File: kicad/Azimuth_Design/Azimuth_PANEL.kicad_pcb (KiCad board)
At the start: 4 copper layers, 101 x 58 mm, 344 parts, among them IC1 BNO086, J1 TYPE-C 16PIN 2MD(073), Q1 LP0404N3T5G, Q2 AO3400A, Q3 AO3401A, U1 ESP32-C3-WROOM-02-N4(4MB), U2 TLV75733PDBVR, U3 TP4054_C5381776

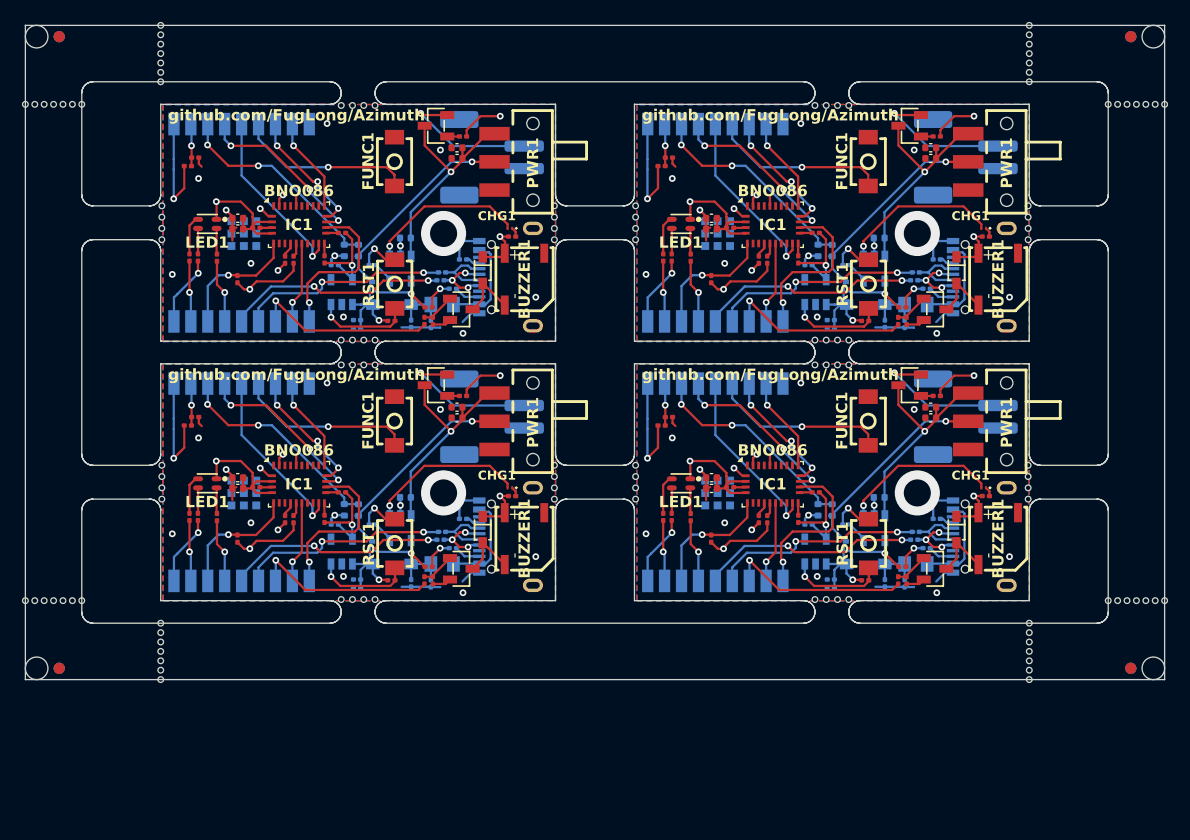
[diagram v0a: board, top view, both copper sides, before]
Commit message: PCB V0.1 ordered!
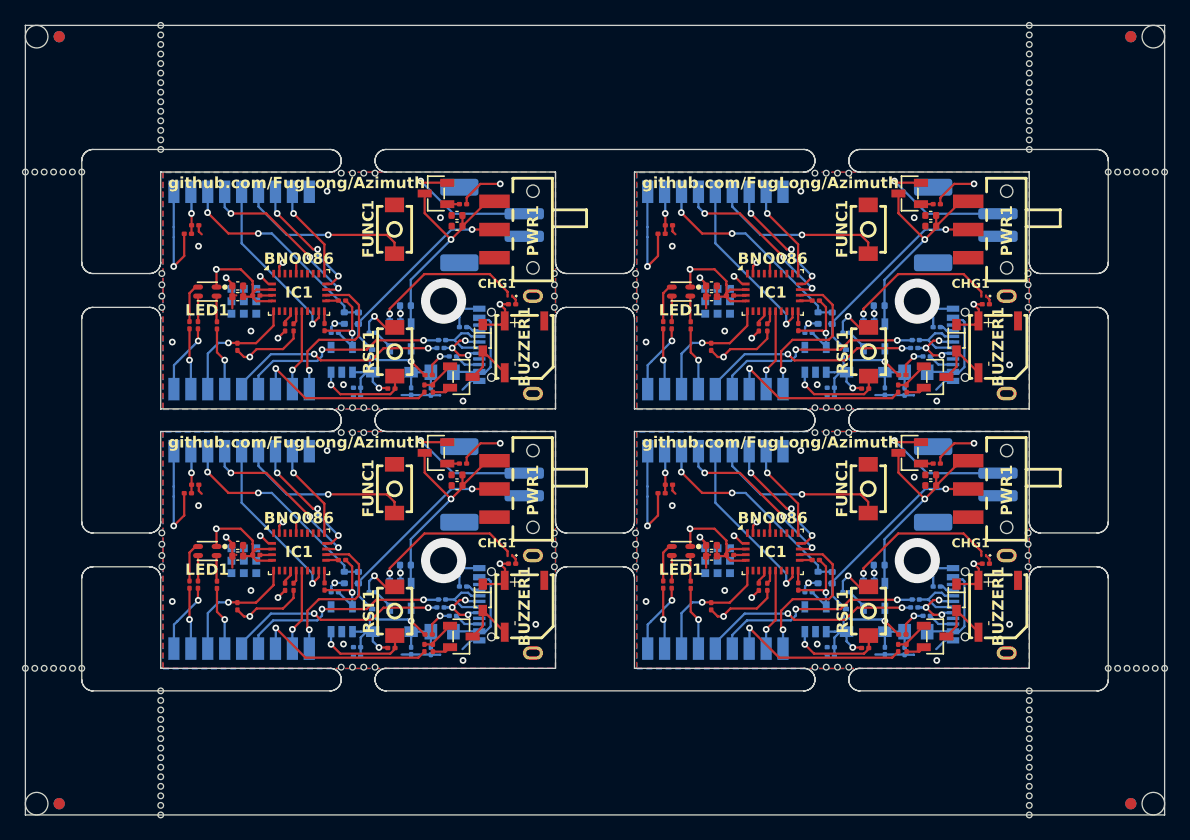
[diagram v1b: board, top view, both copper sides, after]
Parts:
- removed the BUZZER1 at (184.2, 42.5)
- removed the BUZZER1 at (184.2, 65.5)
- removed the BUZZER1 at (142.2, 42.5)
- removed the BUZZER1 at (142.2, 65.5)
- removed the C1 at (136.3, 53.9)
- removed the C1 at (178.3, 30.9)
- removed the C1 at (136.3, 30.9)
- removed the C1 at (178.3, 53.9)
- removed the C10 at (158.8, 61.0)
- removed the C10 at (116.8, 38.0)
- removed the C10 at (158.8, 38.0)
- removed the C10 at (116.8, 61.0)
- removed the C11 at (163.0, 63.8)
- removed the C11 at (121.0, 63.8)
- removed the C11 at (121.0, 40.8)
- removed the C11 at (163.0, 40.8)
- removed the C12 at (113.1, 54.7)
- removed the C12 at (113.1, 31.7)
- removed the C12 at (155.1, 54.7)
- removed the C12 at (155.1, 31.7)
- removed the C2 at (136.3, 31.8)
- removed the C2 at (136.3, 54.8)
- removed the C2 at (178.3, 54.8)
- removed the C2 at (178.3, 31.8)
- removed the C3 at (175.9, 69.5)
- removed the C3 at (133.9, 46.5)
- removed the C3 at (175.9, 46.5)
- removed the C3 at (133.9, 69.5)
- removed the C4 at (127.4, 69.1)
- removed the C4 at (169.4, 46.1)
- removed the C4 at (127.4, 46.1)
- removed the C4 at (169.4, 69.1)
- removed the C5 at (127.4, 46.9)
- removed the C5 at (169.4, 69.9)
- removed the C5 at (169.4, 46.9)
- removed the C5 at (127.4, 69.9)
- removed the C6 at (125.4, 64.2)
- removed the C6 at (125.4, 41.2)
- removed the C6 at (167.4, 41.2)
- removed the C6 at (167.4, 64.2)
- removed the C7 at (133.8, 45.0)
- removed the C7 at (133.8, 68.0)
- removed the C7 at (175.8, 45.0)
- removed the C7 at (175.8, 68.0)
- removed the C8 at (173.7, 38.9)
- removed the C8 at (131.7, 38.9)
- removed the C8 at (131.7, 61.9)
- removed the C8 at (173.7, 61.9)
- removed the C9 at (116.8, 37.1)
- removed the C9 at (116.8, 60.1)
- removed the C9 at (158.8, 37.1)
- removed the C9 at (158.8, 60.1)
- removed the CHG1 at (140.9, 61.0)
- removed the CHG1 at (182.9, 61.0)
- removed the CHG1 at (140.9, 38.0)
- removed the CHG1 at (182.9, 38.0)
- removed the D1 at (172.5, 44.8)
- removed the D1 at (130.5, 67.8)
- removed the D1 at (130.5, 44.8)
- removed the D1 at (172.5, 67.8)
- removed the D2 at (180.6, 64.7)
- removed the D2 at (138.6, 41.7)
- removed the D2 at (138.6, 64.7)
- removed the D2 at (180.6, 41.7)
- removed the F1 at (134.9, 44.8)
- removed the F1 at (176.9, 67.8)
- removed the F1 at (176.9, 44.8)
- removed the F1 at (134.9, 67.8)
- removed the FUNC1 at (130.7, 32.1)
- removed the FUNC1 at (172.7, 55.1)
- removed the FUNC1 at (172.7, 32.1)
- removed the FUNC1 at (130.7, 55.1)
- removed the G*** at (171.1, 55.7)
- removed the G*** at (129.1, 32.7)
- removed the G*** at (171.1, 32.7)
- removed the G*** at (129.1, 55.7)
- removed the IC1 at (164.3, 37.7)
- removed the IC1 at (164.3, 60.7)
- removed the IC1 at (122.3, 37.7)
- removed the IC1 at (122.3, 60.7)
- removed the J1 at (140.6, 42.3)
- removed the J1 at (182.6, 65.3)
- removed the J1 at (182.6, 42.3)
- removed the J1 at (140.6, 65.3)
- removed the LED1 at (156.1, 37.6)
- removed the LED1 at (114.1, 37.6)
- removed the LED1 at (114.1, 60.6)
- removed the LED1 at (156.1, 60.6)
- removed the PH2.0 at (181.4, 54.7)
- removed the PH2.0 at (139.4, 54.7)
- removed the PH2.0 at (181.4, 31.7)
- removed the PH2.0 at (139.4, 31.7)
- removed the PWR1 at (139.6, 32.1)
- removed the PWR1 at (181.6, 55.1)
- removed the PWR1 at (181.6, 32.1)
- removed the PWR1 at (139.6, 55.1)
- removed the Q1 at (128.8, 43.1)
- removed the Q1 at (170.8, 66.1)
- removed the Q1 at (170.8, 43.1)
- removed the Q1 at (128.8, 66.1)
- removed the Q2 at (178.7, 68.2)
- removed the Q2 at (178.7, 45.2)
- removed the Q2 at (136.7, 68.2)
- removed the Q2 at (136.7, 45.2)
- removed the Q3 at (176.4, 51.9)
- removed the Q3 at (134.4, 51.9)
- removed the Q3 at (134.4, 28.9)
- removed the Q3 at (176.4, 28.9)
- removed the R1 at (168.3, 40.0)
- removed the R1 at (168.3, 63.0)
- removed the R1 at (126.3, 63.0)
- removed the R1 at (126.3, 40.0)
- removed the R10 at (135.9, 66.3)
- removed the R10 at (135.9, 43.4)
- removed the R10 at (177.9, 43.4)
- removed the R10 at (177.9, 66.3)
- removed the R11 at (176.8, 42.6)
- removed the R11 at (134.8, 42.6)
- removed the R11 at (176.8, 65.6)
- removed the R11 at (134.8, 65.6)
- removed the R12 at (176.9, 41.9)
- removed the R12 at (176.9, 64.9)
- removed the R12 at (134.9, 64.9)
- removed the R12 at (134.9, 41.9)
- removed the R13 at (118.5, 38.0)
- removed the R13 at (118.5, 61.0)
- removed the R13 at (160.5, 38.0)
- removed the R13 at (160.5, 61.0)
- removed the R14 at (116.8, 65.5)
- removed the R14 at (158.8, 42.5)
- removed the R14 at (116.8, 42.5)
- removed the R14 at (158.8, 65.5)
- removed the R15 at (121.8, 63.8)
- removed the R15 at (163.8, 40.8)
- removed the R15 at (121.8, 40.8)
- removed the R15 at (163.8, 63.8)
- removed the R16 at (166.5, 40.8)
- removed the R16 at (166.5, 63.8)
- removed the R16 at (124.5, 63.8)
- removed the R16 at (124.5, 40.8)
- removed the R17 at (126.1, 38.4)
- removed the R17 at (168.1, 38.4)
- removed the R17 at (126.1, 61.4)
- removed the R17 at (168.1, 61.4)
- removed the R18 at (154.4, 32.5)
- removed the R18 at (112.4, 55.5)
- removed the R18 at (154.4, 55.5)
- removed the R18 at (112.4, 32.5)
- removed the R19 at (172.4, 69.2)
- removed the R19 at (172.4, 46.2)
- removed the R19 at (130.4, 46.2)
- removed the R19 at (130.4, 69.2)
- removed the R2 at (169.5, 40.0)
- removed the R2 at (169.5, 63.0)
- removed the R2 at (127.5, 63.0)
- removed the R2 at (127.5, 40.0)
- removed the R20 at (175.4, 46.2)
- removed the R20 at (133.4, 46.2)
- removed the R20 at (175.4, 69.2)
- removed the R20 at (133.4, 69.2)
- removed the R21 at (176.1, 46.2)
- removed the R21 at (134.1, 69.2)
- removed the R21 at (176.1, 69.2)
- removed the R21 at (134.1, 46.2)
- removed the R22 at (136.8, 29.9)
- removed the R22 at (178.8, 29.9)
- removed the R22 at (136.8, 52.9)
- removed the R22 at (178.8, 52.9)
- removed the R3 at (132.2, 69.5)
- removed the R3 at (174.2, 46.5)
- removed the R3 at (132.2, 46.5)
- removed the R3 at (174.2, 69.5)
- removed the R4 at (170.8, 41.2)
- removed the R4 at (128.8, 41.2)
- removed the R4 at (170.8, 64.2)
- removed the R4 at (128.8, 64.2)
- removed the R5 at (183.2, 38.7)
- removed the R5 at (183.2, 61.7)
- removed the R5 at (141.2, 61.7)
- removed the R5 at (141.2, 38.7)
- removed the R6 at (157.0, 40.6)
- removed the R6 at (115.0, 40.6)
- removed the R6 at (115.0, 63.6)
- removed the R6 at (157.0, 63.6)
- removed the R7 at (113.3, 40.6)
- removed the R7 at (155.3, 40.6)
- removed the R7 at (113.3, 63.6)
- removed the R7 at (155.3, 63.6)
- removed the R8 at (112.5, 40.6)
- removed the R8 at (112.5, 63.6)
- removed the R8 at (154.6, 63.6)
- removed the R8 at (154.6, 40.6)
- removed the R9 at (178.8, 40.8)
- removed the R9 at (136.8, 40.8)
- removed the R9 at (136.8, 63.8)
- removed the R9 at (178.8, 63.8)
- removed the RST1 at (130.8, 65.9)
- removed the RST1 at (130.8, 42.9)
- removed the RST1 at (172.8, 42.9)
- removed the RST1 at (172.8, 65.9)
- removed the U1 at (117.2, 60.5)
- removed the U1 at (159.2, 37.5)
- removed the U1 at (117.2, 37.5)
- removed the U1 at (159.2, 60.5)
- removed the U2 at (168.1, 43.6)
- removed the U2 at (126.0, 66.7)
- removed the U2 at (168.1, 66.7)
- removed the U2 at (126.0, 43.6)
- removed the U3 at (173.2, 41.6)
- removed the U3 at (131.2, 64.6)
- removed the U3 at (173.2, 64.6)
- removed the U3 at (131.2, 41.6)
- added BUZZER1: MLT-5020, 1_MyFootPrints:BUZ-SMD_L5.0-W5.5-P4.60, F.Cu at (184.2, 71.5)
- added BUZZER1: MLT-5020, 1_MyFootPrints:BUZ-SMD_L5.0-W5.5-P4.60, F.Cu at (184.2, 48.5)
- added BUZZER1: MLT-5020, 1_MyFootPrints:BUZ-SMD_L5.0-W5.5-P4.60, F.Cu at (142.2, 71.5)
- added BUZZER1: MLT-5020, 1_MyFootPrints:BUZ-SMD_L5.0-W5.5-P4.60, F.Cu at (142.2, 48.5)
- added C1: 10uf, Capacitor_SMD:C_0402_1005Metric, F.Cu at (178.3, 36.9)
- added C1: 10uf, Capacitor_SMD:C_0402_1005Metric, F.Cu at (136.3, 36.9)
- added C1: 10uf, Capacitor_SMD:C_0402_1005Metric, F.Cu at (136.3, 59.9)
- added C1: 10uf, Capacitor_SMD:C_0402_1005Metric, F.Cu at (178.3, 59.9)
- added C10: 0.1uf, Capacitor_SMD:C_0402_1005Metric, F.Cu at (158.8, 44.0)
- added C10: 0.1uf, Capacitor_SMD:C_0402_1005Metric, F.Cu at (116.8, 67.0)
- added C10: 0.1uf, Capacitor_SMD:C_0402_1005Metric, F.Cu at (116.8, 44.0)
- added C10: 0.1uf, Capacitor_SMD:C_0402_1005Metric, F.Cu at (158.8, 67.0)
- added C11: 100nf, Capacitor_SMD:C_0201_0603Metric, F.Cu at (163.0, 46.8)
- added C11: 100nf, Capacitor_SMD:C_0201_0603Metric, F.Cu at (121.0, 69.8)
- added C11: 100nf, Capacitor_SMD:C_0201_0603Metric, F.Cu at (163.0, 69.8)
- added C11: 100nf, Capacitor_SMD:C_0201_0603Metric, F.Cu at (121.0, 46.8)
- added C12: 100nf, Capacitor_SMD:C_0201_0603Metric, F.Cu at (155.1, 37.7)
- added C12: 100nf, Capacitor_SMD:C_0201_0603Metric, F.Cu at (155.1, 60.7)
- added C12: 100nf, Capacitor_SMD:C_0201_0603Metric, F.Cu at (113.1, 60.7)
- added C12: 100nf, Capacitor_SMD:C_0201_0603Metric, F.Cu at (113.1, 37.7)
- added C2: 0.1uf, Capacitor_SMD:C_0402_1005Metric, F.Cu at (178.3, 37.8)
- added C2: 0.1uf, Capacitor_SMD:C_0402_1005Metric, F.Cu at (136.3, 60.8)
- added C2: 0.1uf, Capacitor_SMD:C_0402_1005Metric, F.Cu at (178.3, 60.8)
- added C2: 0.1uf, Capacitor_SMD:C_0402_1005Metric, F.Cu at (136.3, 37.8)
- added C3: 100nf, Capacitor_SMD:C_0201_0603Metric, B.Cu at (175.9, 52.5)
- added C3: 100nf, Capacitor_SMD:C_0201_0603Metric, B.Cu at (133.9, 52.5)
- added C3: 100nf, Capacitor_SMD:C_0201_0603Metric, B.Cu at (175.9, 75.5)
- added C3: 100nf, Capacitor_SMD:C_0201_0603Metric, B.Cu at (133.9, 75.5)
- added C4: 2.2uf, Capacitor_SMD:C_0201_0603Metric, B.Cu at (127.4, 52.1)
- added C4: 2.2uf, Capacitor_SMD:C_0201_0603Metric, B.Cu at (169.4, 52.1)
- added C4: 2.2uf, Capacitor_SMD:C_0201_0603Metric, B.Cu at (169.4, 75.1)
- added C4: 2.2uf, Capacitor_SMD:C_0201_0603Metric, B.Cu at (127.4, 75.1)
- added C5: 2.2uf, Capacitor_SMD:C_0201_0603Metric, B.Cu at (127.4, 75.9)
- added C5: 2.2uf, Capacitor_SMD:C_0201_0603Metric, B.Cu at (127.4, 52.9)
- added C5: 2.2uf, Capacitor_SMD:C_0201_0603Metric, B.Cu at (169.4, 52.9)
- added C5: 2.2uf, Capacitor_SMD:C_0201_0603Metric, B.Cu at (169.4, 75.9)
- added C6: 2.2uf, Capacitor_SMD:C_0201_0603Metric, B.Cu at (125.4, 47.2)
- added C6: 2.2uf, Capacitor_SMD:C_0201_0603Metric, B.Cu at (167.4, 70.2)
- added C6: 2.2uf, Capacitor_SMD:C_0201_0603Metric, B.Cu at (125.4, 70.2)
- added C6: 2.2uf, Capacitor_SMD:C_0201_0603Metric, B.Cu at (167.4, 47.2)
- added C7: 2.2uf, Capacitor_SMD:C_0201_0603Metric, F.Cu at (175.8, 74.0)
- added C7: 2.2uf, Capacitor_SMD:C_0201_0603Metric, F.Cu at (175.8, 51.0)
- added C7: 2.2uf, Capacitor_SMD:C_0201_0603Metric, F.Cu at (133.8, 74.0)
- added C7: 2.2uf, Capacitor_SMD:C_0201_0603Metric, F.Cu at (133.8, 51.0)
- added C8: 10uf, Capacitor_SMD:C_0402_1005Metric, B.Cu at (173.7, 67.8)
- added C8: 10uf, Capacitor_SMD:C_0402_1005Metric, B.Cu at (131.7, 44.9)
- added C8: 10uf, Capacitor_SMD:C_0402_1005Metric, B.Cu at (131.7, 67.8)
- added C8: 10uf, Capacitor_SMD:C_0402_1005Metric, B.Cu at (173.7, 44.9)
- added C9: 10uf, Capacitor_SMD:C_0402_1005Metric, F.Cu at (158.8, 43.1)
- added C9: 10uf, Capacitor_SMD:C_0402_1005Metric, F.Cu at (116.8, 66.1)
- added C9: 10uf, Capacitor_SMD:C_0402_1005Metric, F.Cu at (116.8, 43.1)
- added C9: 10uf, Capacitor_SMD:C_0402_1005Metric, F.Cu at (158.8, 66.1)
- added CHG1: XL-0201SURC, 1_MyFootPrints:LED-SMD_L0.65-W0.35-P0.41_XL-0201SURC, F.Cu at (182.9, 44.0)
- added CHG1: XL-0201SURC, 1_MyFootPrints:LED-SMD_L0.65-W0.35-P0.41_XL-0201SURC, F.Cu at (182.9, 67.0)
- added CHG1: XL-0201SURC, 1_MyFootPrints:LED-SMD_L0.65-W0.35-P0.41_XL-0201SURC, F.Cu at (140.9, 67.0)
- added CHG1: XL-0201SURC, 1_MyFootPrints:LED-SMD_L0.65-W0.35-P0.41_XL-0201SURC, F.Cu at (140.9, 44.0)
- added D1: MBR0530_C5204746, 1_MyFootPrints:SOD-123_L2.7-W1.6-LS3.7-RD-1, B.Cu at (172.5, 50.8)
- added D1: MBR0530_C5204746, 1_MyFootPrints:SOD-123_L2.7-W1.6-LS3.7-RD-1, B.Cu at (130.5, 73.8)
- added D1: MBR0530_C5204746, 1_MyFootPrints:SOD-123_L2.7-W1.6-LS3.7-RD-1, B.Cu at (172.5, 73.8)
- added D1: MBR0530_C5204746, 1_MyFootPrints:SOD-123_L2.7-W1.6-LS3.7-RD-1, B.Cu at (130.5, 50.8)
- added D2: B5819WS, 1_MyFootPrints:SOD-323_L1.8-W1.3-LS2.5-RD, F.Cu at (180.6, 70.7)
- added D2: B5819WS, 1_MyFootPrints:SOD-323_L1.8-W1.3-LS2.5-RD, F.Cu at (138.6, 47.7)
- added D2: B5819WS, 1_MyFootPrints:SOD-323_L1.8-W1.3-LS2.5-RD, F.Cu at (180.6, 47.7)
- added D2: B5819WS, 1_MyFootPrints:SOD-323_L1.8-W1.3-LS2.5-RD, F.Cu at (138.6, 70.7)
- added F1: 0805L050WR, 1_MyFootPrints:R0805, B.Cu at (176.9, 73.8)
- added F1: 0805L050WR, 1_MyFootPrints:R0805, B.Cu at (176.9, 50.8)
- added F1: 0805L050WR, 1_MyFootPrints:R0805, B.Cu at (134.9, 73.8)
- added F1: 0805L050WR, 1_MyFootPrints:R0805, B.Cu at (134.9, 50.8)
- added FUNC1: HX 3X4X2-2P-1.6N TACTILE SWITCH, 1_MyFootPrints:KEY-SMD_L4.0-W3.0-LS4.9-1, F.Cu at (172.7, 38.1)
- added FUNC1: HX 3X4X2-2P-1.6N TACTILE SWITCH, 1_MyFootPrints:KEY-SMD_L4.0-W3.0-LS4.9-1, F.Cu at (130.7, 61.1)
- added FUNC1: HX 3X4X2-2P-1.6N TACTILE SWITCH, 1_MyFootPrints:KEY-SMD_L4.0-W3.0-LS4.9-1, F.Cu at (130.7, 38.1)
- added FUNC1: HX 3X4X2-2P-1.6N TACTILE SWITCH, 1_MyFootPrints:KEY-SMD_L4.0-W3.0-LS4.9-1, F.Cu at (172.7, 61.1)
- added G***: LOGO, LOGO, B.Cu at (129.1, 38.7)
- added G***: LOGO, LOGO, B.Cu at (129.1, 61.7)
- added G***: LOGO, LOGO, B.Cu at (171.1, 38.7)
- added G***: LOGO, LOGO, B.Cu at (171.1, 61.7)
- added IC1: BNO086, Package_LGA:LGA-28_5.2x3.8mm_P0.5mm, F.Cu at (164.3, 66.7)
- added IC1: BNO086, Package_LGA:LGA-28_5.2x3.8mm_P0.5mm, F.Cu at (122.3, 43.7)
- added IC1: BNO086, Package_LGA:LGA-28_5.2x3.8mm_P0.5mm, F.Cu at (122.3, 66.7)
- added IC1: BNO086, Package_LGA:LGA-28_5.2x3.8mm_P0.5mm, F.Cu at (164.3, 43.7)
- added J1: TYPE-C 16PIN 2MD(073), 1_MyFootPrints:USB-C-SMD_TYPE-C-6PIN-2MD-073, B.Cu at (140.6, 71.3)
- added J1: TYPE-C 16PIN 2MD(073), 1_MyFootPrints:USB-C-SMD_TYPE-C-6PIN-2MD-073, B.Cu at (182.6, 48.3)
- added J1: TYPE-C 16PIN 2MD(073), 1_MyFootPrints:USB-C-SMD_TYPE-C-6PIN-2MD-073, B.Cu at (182.6, 71.3)
- added J1: TYPE-C 16PIN 2MD(073), 1_MyFootPrints:USB-C-SMD_TYPE-C-6PIN-2MD-073, B.Cu at (140.6, 48.3)
- added KiKit_MB_17_10: NPTH, NPTH, F.Cu at (110.0, 27.6)
- added KiKit_MB_17_11: NPTH, NPTH, F.Cu at (110.0, 28.5)
- added KiKit_MB_17_12: NPTH, NPTH, F.Cu at (110.0, 29.3)
- added KiKit_MB_17_13: NPTH, NPTH, F.Cu at (110.0, 30.2)
- added KiKit_MB_17_14: NPTH, NPTH, F.Cu at (110.0, 31.0)
- added KiKit_MB_17_8: NPTH, NPTH, F.Cu at (110.0, 25.9)
- added KiKit_MB_17_9: NPTH, NPTH, F.Cu at (110.0, 26.8)
- added KiKit_MB_18_10: NPTH, NPTH, F.Cu at (187.0, 27.6)
- added KiKit_MB_18_11: NPTH, NPTH, F.Cu at (187.0, 28.5)
- added KiKit_MB_18_12: NPTH, NPTH, F.Cu at (187.0, 29.3)
- added KiKit_MB_18_13: NPTH, NPTH, F.Cu at (187.0, 30.2)
- added KiKit_MB_18_14: NPTH, NPTH, F.Cu at (187.0, 31.0)
- added KiKit_MB_18_8: NPTH, NPTH, F.Cu at (187.0, 25.9)
- added KiKit_MB_18_9: NPTH, NPTH, F.Cu at (187.0, 26.8)
- added KiKit_MB_19_10: NPTH, NPTH, F.Cu at (110.0, 86.6)
- added KiKit_MB_19_11: NPTH, NPTH, F.Cu at (110.0, 87.5)
- added KiKit_MB_19_12: NPTH, NPTH, F.Cu at (110.0, 88.3)
- added KiKit_MB_19_13: NPTH, NPTH, F.Cu at (110.0, 89.2)
- added KiKit_MB_19_14: NPTH, NPTH, F.Cu at (110.0, 90.0)
- added KiKit_MB_19_8: NPTH, NPTH, F.Cu at (110.0, 84.9)
- added KiKit_MB_19_9: NPTH, NPTH, F.Cu at (110.0, 85.8)
- added KiKit_MB_20_10: NPTH, NPTH, F.Cu at (187.0, 86.6)
- added KiKit_MB_20_11: NPTH, NPTH, F.Cu at (187.0, 87.5)
- added KiKit_MB_20_12: NPTH, NPTH, F.Cu at (187.0, 88.3)
- added KiKit_MB_20_13: NPTH, NPTH, F.Cu at (187.0, 89.2)
- added KiKit_MB_20_14: NPTH, NPTH, F.Cu at (187.0, 90.0)
- added KiKit_MB_20_8: NPTH, NPTH, F.Cu at (187.0, 84.9)
- added KiKit_MB_20_9: NPTH, NPTH, F.Cu at (187.0, 85.8)
- added LED1: TZ-P4-1615RGBTCA1-0.55T, rgb_led_C779813:LED-SMD_4P-L1.6-W1.5-BR_TZ-P4-1615, F.Cu at (156.1, 66.6)
- added LED1: TZ-P4-1615RGBTCA1-0.55T, rgb_led_C779813:LED-SMD_4P-L1.6-W1.5-BR_TZ-P4-1615, F.Cu at (114.1, 43.6)
- added LED1: TZ-P4-1615RGBTCA1-0.55T, rgb_led_C779813:LED-SMD_4P-L1.6-W1.5-BR_TZ-P4-1615, F.Cu at (156.1, 43.6)
- added LED1: TZ-P4-1615RGBTCA1-0.55T, rgb_led_C779813:LED-SMD_4P-L1.6-W1.5-BR_TZ-P4-1615, F.Cu at (114.1, 66.6)
- added PH2.0: S2B-PH-SM4-TB(LF)(SN), Connector_JST:JST_PH_S2B-PH-SM4-TB_1x02-1MP_P2.00mm_Horizontal, B.Cu at (181.4, 37.7)
- added PH2.0: S2B-PH-SM4-TB(LF)(SN), Connector_JST:JST_PH_S2B-PH-SM4-TB_1x02-1MP_P2.00mm_Horizontal, B.Cu at (139.4, 60.7)
- added PH2.0: S2B-PH-SM4-TB(LF)(SN), Connector_JST:JST_PH_S2B-PH-SM4-TB_1x02-1MP_P2.00mm_Horizontal, B.Cu at (139.4, 37.7)
- added PH2.0: S2B-PH-SM4-TB(LF)(SN), Connector_JST:JST_PH_S2B-PH-SM4-TB_1x02-1MP_P2.00mm_Horizontal, B.Cu at (181.4, 60.7)
- added PWR1: K3-1280S-K1, 1_MyFootPrints:SW-SMD_K3-1280S-K1, F.Cu at (181.6, 61.1)
- added PWR1: K3-1280S-K1, 1_MyFootPrints:SW-SMD_K3-1280S-K1, F.Cu at (139.6, 38.1)
- added PWR1: K3-1280S-K1, 1_MyFootPrints:SW-SMD_K3-1280S-K1, F.Cu at (181.6, 38.1)
- added PWR1: K3-1280S-K1, 1_MyFootPrints:SW-SMD_K3-1280S-K1, F.Cu at (139.6, 61.1)
- added Q1: LP0404N3T5G, 1_MyFootPrints:SOT-883-3_L1.0-W0.6-BR, B.Cu at (128.8, 72.1)
- added Q1: LP0404N3T5G, 1_MyFootPrints:SOT-883-3_L1.0-W0.6-BR, B.Cu at (128.8, 49.1)
- added Q1: LP0404N3T5G, 1_MyFootPrints:SOT-883-3_L1.0-W0.6-BR, B.Cu at (170.8, 49.1)
- added Q1: LP0404N3T5G, 1_MyFootPrints:SOT-883-3_L1.0-W0.6-BR, B.Cu at (170.8, 72.1)
- added Q2: AO3400A, 1_MyFootPrints:SOT-23-3_L2.9-W1.3-P1.90-LS2.4-BR, F.Cu at (178.7, 74.2)
- added Q2: AO3400A, 1_MyFootPrints:SOT-23-3_L2.9-W1.3-P1.90-LS2.4-BR, F.Cu at (178.7, 51.2)
- added Q2: AO3400A, 1_MyFootPrints:SOT-23-3_L2.9-W1.3-P1.90-LS2.4-BR, F.Cu at (136.7, 74.2)
- added Q2: AO3400A, 1_MyFootPrints:SOT-23-3_L2.9-W1.3-P1.90-LS2.4-BR, F.Cu at (136.7, 51.2)
- added Q3: AO3401A, 1_MyFootPrints:SOT-23-3_L2.9-W1.3-P1.90-LS2.4-BR, F.Cu at (176.4, 57.9)
- added Q3: AO3401A, 1_MyFootPrints:SOT-23-3_L2.9-W1.3-P1.90-LS2.4-BR, F.Cu at (134.4, 34.9)
- added Q3: AO3401A, 1_MyFootPrints:SOT-23-3_L2.9-W1.3-P1.90-LS2.4-BR, F.Cu at (134.4, 57.9)
- added Q3: AO3401A, 1_MyFootPrints:SOT-23-3_L2.9-W1.3-P1.90-LS2.4-BR, F.Cu at (176.4, 34.9)
- added R1: 220k, Resistor_SMD:R_0402_1005Metric, B.Cu at (126.3, 69.0)
- added R1: 220k, Resistor_SMD:R_0402_1005Metric, B.Cu at (126.3, 46.0)
- added R1: 220k, Resistor_SMD:R_0402_1005Metric, B.Cu at (168.3, 46.0)
- added R1: 220k, Resistor_SMD:R_0402_1005Metric, B.Cu at (168.3, 69.0)
- added R10: 5.1k, Resistor_SMD:R_0201_0603Metric, B.Cu at (135.9, 72.3)
- added R10: 5.1k, Resistor_SMD:R_0201_0603Metric, B.Cu at (177.9, 72.3)
- added R10: 5.1k, Resistor_SMD:R_0201_0603Metric, B.Cu at (135.9, 49.4)
- added R10: 5.1k, Resistor_SMD:R_0201_0603Metric, B.Cu at (177.9, 49.4)
- added R11: 22R, Resistor_SMD:R_0201_0603Metric, B.Cu at (134.8, 71.6)
- added R11: 22R, Resistor_SMD:R_0201_0603Metric, B.Cu at (176.8, 71.6)
- added R11: 22R, Resistor_SMD:R_0201_0603Metric, B.Cu at (176.8, 48.6)
- added R11: 22R, Resistor_SMD:R_0201_0603Metric, B.Cu at (134.8, 48.6)
- added R12: 22R, Resistor_SMD:R_0201_0603Metric, B.Cu at (176.9, 47.9)
- added R12: 22R, Resistor_SMD:R_0201_0603Metric, B.Cu at (176.9, 70.9)
- added R12: 22R, Resistor_SMD:R_0201_0603Metric, B.Cu at (134.9, 47.9)
- added R12: 22R, Resistor_SMD:R_0201_0603Metric, B.Cu at (134.9, 70.9)
- added R13: 10k, Resistor_SMD:R_0201_0603Metric, F.Cu at (160.5, 44.0)
- added R13: 10k, Resistor_SMD:R_0201_0603Metric, F.Cu at (118.5, 67.0)
- added R13: 10k, Resistor_SMD:R_0201_0603Metric, F.Cu at (118.5, 44.0)
- added R13: 10k, Resistor_SMD:R_0201_0603Metric, F.Cu at (160.5, 67.0)
- added R14: 10k, Resistor_SMD:R_0201_0603Metric, F.Cu at (158.8, 71.5)
- added R14: 10k, Resistor_SMD:R_0201_0603Metric, F.Cu at (116.8, 48.5)
- added R14: 10k, Resistor_SMD:R_0201_0603Metric, F.Cu at (158.8, 48.5)
- added R14: 10k, Resistor_SMD:R_0201_0603Metric, F.Cu at (116.8, 71.5)
- added R15: 10k, Resistor_SMD:R_0201_0603Metric, F.Cu at (121.8, 69.8)
- added R15: 10k, Resistor_SMD:R_0201_0603Metric, F.Cu at (163.8, 46.8)
- added R15: 10k, Resistor_SMD:R_0201_0603Metric, F.Cu at (121.8, 46.8)
- added R15: 10k, Resistor_SMD:R_0201_0603Metric, F.Cu at (163.8, 69.8)
- added R16: 4.7k, Resistor_SMD:R_0201_0603Metric, F.Cu at (166.5, 69.8)
- added R16: 4.7k, Resistor_SMD:R_0201_0603Metric, F.Cu at (124.5, 46.8)
- added R16: 4.7k, Resistor_SMD:R_0201_0603Metric, F.Cu at (166.5, 46.8)
- added R16: 4.7k, Resistor_SMD:R_0201_0603Metric, F.Cu at (124.5, 69.8)
- added R17: 4.7k, Resistor_SMD:R_0201_0603Metric, F.Cu at (168.1, 67.4)
- added R17: 4.7k, Resistor_SMD:R_0201_0603Metric, F.Cu at (168.1, 44.4)
- added R17: 4.7k, Resistor_SMD:R_0201_0603Metric, F.Cu at (126.1, 44.4)
- added R17: 4.7k, Resistor_SMD:R_0201_0603Metric, F.Cu at (126.1, 67.4)
- added R18: 10k, Resistor_SMD:R_0201_0603Metric, F.Cu at (154.4, 61.5)
- added R18: 10k, Resistor_SMD:R_0201_0603Metric, F.Cu at (112.4, 61.5)
- added R18: 10k, Resistor_SMD:R_0201_0603Metric, F.Cu at (112.4, 38.5)
- added R18: 10k, Resistor_SMD:R_0201_0603Metric, F.Cu at (154.4, 38.5)
- added R19: 10k, Resistor_SMD:R_0201_0603Metric, F.Cu at (172.4, 75.2)
- added R19: 10k, Resistor_SMD:R_0201_0603Metric, F.Cu at (130.4, 75.2)
- added R19: 10k, Resistor_SMD:R_0201_0603Metric, F.Cu at (172.4, 52.2)
- added R19: 10k, Resistor_SMD:R_0201_0603Metric, F.Cu at (130.4, 52.2)
- added R2: 220k, Resistor_SMD:R_0402_1005Metric, B.Cu at (169.5, 46.0)
- added R2: 220k, Resistor_SMD:R_0402_1005Metric, B.Cu at (127.5, 46.0)
- added R2: 220k, Resistor_SMD:R_0402_1005Metric, B.Cu at (169.5, 69.0)
- added R2: 220k, Resistor_SMD:R_0402_1005Metric, B.Cu at (127.5, 69.0)
- added R20: 330R, Resistor_SMD:R_0201_0603Metric, F.Cu at (175.4, 52.2)
- added R20: 330R, Resistor_SMD:R_0201_0603Metric, F.Cu at (175.4, 75.2)
- added R20: 330R, Resistor_SMD:R_0201_0603Metric, F.Cu at (133.4, 52.2)
- added R20: 330R, Resistor_SMD:R_0201_0603Metric, F.Cu at (133.4, 75.2)
- added R21: 100k, Resistor_SMD:R_0201_0603Metric, F.Cu at (176.1, 52.2)
- added R21: 100k, Resistor_SMD:R_0201_0603Metric, F.Cu at (134.1, 52.2)
- added R21: 100k, Resistor_SMD:R_0201_0603Metric, F.Cu at (176.1, 75.2)
- added R21: 100k, Resistor_SMD:R_0201_0603Metric, F.Cu at (134.1, 75.2)
- added R22: 100k, Resistor_SMD:R_0201_0603Metric, F.Cu at (136.8, 35.9)
- added R22: 100k, Resistor_SMD:R_0201_0603Metric, F.Cu at (136.8, 58.9)
- added R22: 100k, Resistor_SMD:R_0201_0603Metric, F.Cu at (178.8, 35.9)
- added R22: 100k, Resistor_SMD:R_0201_0603Metric, F.Cu at (178.8, 58.9)
- added R3: 100k, Resistor_SMD:R_0201_0603Metric, B.Cu at (132.2, 75.5)
- added R3: 100k, Resistor_SMD:R_0201_0603Metric, B.Cu at (132.2, 52.5)
- added R3: 100k, Resistor_SMD:R_0201_0603Metric, B.Cu at (174.2, 75.5)
- added R3: 100k, Resistor_SMD:R_0201_0603Metric, B.Cu at (174.2, 52.5)
- added R4: 2K, Resistor_SMD:R_0201_0603Metric, B.Cu at (128.8, 70.2)
- added R4: 2K, Resistor_SMD:R_0201_0603Metric, B.Cu at (170.8, 47.2)
- added R4: 2K, Resistor_SMD:R_0201_0603Metric, B.Cu at (128.8, 47.2)
- added R4: 2K, Resistor_SMD:R_0201_0603Metric, B.Cu at (170.8, 70.2)
- added R5: 150R, Resistor_SMD:R_0201_0603Metric, F.Cu at (183.2, 67.7)
- added R5: 150R, Resistor_SMD:R_0201_0603Metric, F.Cu at (141.2, 67.7)
- added R5: 150R, Resistor_SMD:R_0201_0603Metric, F.Cu at (183.2, 44.7)
- added R5: 150R, Resistor_SMD:R_0201_0603Metric, F.Cu at (141.2, 44.7)
- added R6: 220R, Resistor_SMD:R_0201_0603Metric, F.Cu at (115.0, 46.6)
- added R6: 220R, Resistor_SMD:R_0201_0603Metric, F.Cu at (157.0, 46.6)
- added R6: 220R, Resistor_SMD:R_0201_0603Metric, F.Cu at (115.0, 69.6)
- added R6: 220R, Resistor_SMD:R_0201_0603Metric, F.Cu at (157.0, 69.6)
- added R7: 100R, Resistor_SMD:R_0201_0603Metric, F.Cu at (155.3, 69.6)
- added R7: 100R, Resistor_SMD:R_0201_0603Metric, F.Cu at (113.3, 69.6)
- added R7: 100R, Resistor_SMD:R_0201_0603Metric, F.Cu at (113.3, 46.6)
- added R7: 100R, Resistor_SMD:R_0201_0603Metric, F.Cu at (155.3, 46.6)
- added R8: 68R, Resistor_SMD:R_0201_0603Metric, F.Cu at (112.5, 69.6)
- added R8: 68R, Resistor_SMD:R_0201_0603Metric, F.Cu at (112.5, 46.6)
- added R8: 68R, Resistor_SMD:R_0201_0603Metric, F.Cu at (154.6, 46.6)
- added R8: 68R, Resistor_SMD:R_0201_0603Metric, F.Cu at (154.6, 69.6)
- added R9: 5.1k, Resistor_SMD:R_0201_0603Metric, B.Cu at (178.8, 46.8)
- added R9: 5.1k, Resistor_SMD:R_0201_0603Metric, B.Cu at (178.8, 69.8)
- added R9: 5.1k, Resistor_SMD:R_0201_0603Metric, B.Cu at (136.8, 46.8)
- added R9: 5.1k, Resistor_SMD:R_0201_0603Metric, B.Cu at (136.8, 69.8)
- added RST1: HX 3X4X2-2P-1.6N TACTILE SWITCH, 1_MyFootPrints:KEY-SMD_L4.0-W3.0-LS4.9-1, F.Cu at (172.8, 48.9)
- added RST1: HX 3X4X2-2P-1.6N TACTILE SWITCH, 1_MyFootPrints:KEY-SMD_L4.0-W3.0-LS4.9-1, F.Cu at (130.8, 48.9)
- added RST1: HX 3X4X2-2P-1.6N TACTILE SWITCH, 1_MyFootPrints:KEY-SMD_L4.0-W3.0-LS4.9-1, F.Cu at (172.8, 71.9)
- added RST1: HX 3X4X2-2P-1.6N TACTILE SWITCH, 1_MyFootPrints:KEY-SMD_L4.0-W3.0-LS4.9-1, F.Cu at (130.8, 71.9)
- added U1: ESP32-C3-WROOM-02-N4(4MB), 1_MyFootPrints:BULETM-SMD_ESPRESSIF_ESP32-C3-WROOM-02-N4-4MB, B.Cu at (117.2, 43.5)
- added U1: ESP32-C3-WROOM-02-N4(4MB), 1_MyFootPrints:BULETM-SMD_ESPRESSIF_ESP32-C3-WROOM-02-N4-4MB, B.Cu at (117.2, 66.5)
- added U1: ESP32-C3-WROOM-02-N4(4MB), 1_MyFootPrints:BULETM-SMD_ESPRESSIF_ESP32-C3-WROOM-02-N4-4MB, B.Cu at (159.2, 43.5)
- added U1: ESP32-C3-WROOM-02-N4(4MB), 1_MyFootPrints:BULETM-SMD_ESPRESSIF_ESP32-C3-WROOM-02-N4-4MB, B.Cu at (159.2, 66.5)
- added U2: TLV75733PDBVR, 1_MyFootPrints:SOT-23-5_L2.9-W1.6-P0.95-LS2.8-BL, B.Cu at (168.1, 72.7)
- added U2: TLV75733PDBVR, 1_MyFootPrints:SOT-23-5_L2.9-W1.6-P0.95-LS2.8-BL, B.Cu at (168.1, 49.6)
- added U2: TLV75733PDBVR, 1_MyFootPrints:SOT-23-5_L2.9-W1.6-P0.95-LS2.8-BL, B.Cu at (126.0, 72.7)
- added U2: TLV75733PDBVR, 1_MyFootPrints:SOT-23-5_L2.9-W1.6-P0.95-LS2.8-BL, B.Cu at (126.0, 49.6)
- added U3: TP4054_C5381776, 1_MyFootPrints:SOT-23-5_L2.9-W1.6-P0.95-LS2.8-BR, B.Cu at (173.2, 47.6)
- added U3: TP4054_C5381776, 1_MyFootPrints:SOT-23-5_L2.9-W1.6-P0.95-LS2.8-BR, B.Cu at (131.2, 47.6)
- added U3: TP4054_C5381776, 1_MyFootPrints:SOT-23-5_L2.9-W1.6-P0.95-LS2.8-BR, B.Cu at (173.2, 70.6)
- added U3: TP4054_C5381776, 1_MyFootPrints:SOT-23-5_L2.9-W1.6-P0.95-LS2.8-BR, B.Cu at (131.2, 70.6)
- moved KiKit_FID_B_3 12.0 mm to (101.0, 89.0)
- moved KiKit_FID_B_4 12.0 mm to (196.0, 89.0)
- moved KiKit_FID_T_3 12.0 mm to (101.0, 89.0)
- moved KiKit_FID_T_4 12.0 mm to (196.0, 89.0)
- moved KiKit_TO_3 12.0 mm to (99.0, 89.0)
- moved KiKit_TO_4 12.0 mm to (198.0, 89.0)
- moved KiKit_MB_19_7 6.08 mm to (110.0, 84.1)
- moved KiKit_MB_20_7 6.08 mm to (187.0, 84.1)
- moved KiKit_MB_19_6 6.06 mm to (110.0, 83.2)
- moved KiKit_MB_20_6 6.06 mm to (187.0, 83.2)
- moved KiKit_MB_19_5 6.05 mm to (110.0, 82.4)
- moved KiKit_MB_20_5 6.05 mm to (187.0, 82.4)
- moved KiKit_MB_19_4 6.04 mm to (110.0, 81.5)
- moved KiKit_MB_20_4 6.04 mm to (187.0, 81.5)
- moved KiKit_MB_19_3 6.03 mm to (110.0, 80.7)
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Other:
- board size 101 x 58 mm -> 101 x 70 mm
